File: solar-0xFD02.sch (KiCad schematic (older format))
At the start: 25 parts, among them J1 Solar, J2 BAT, J3 ESP32, Q1 MOSFET, U1 CN3801

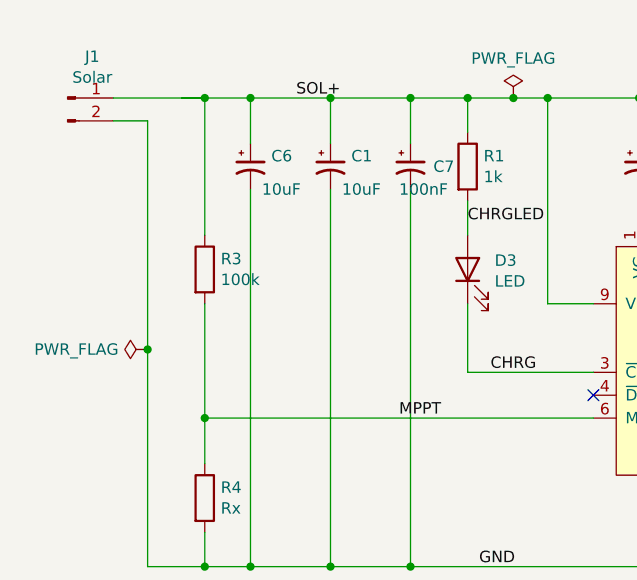
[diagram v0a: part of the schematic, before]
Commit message: Cleanup
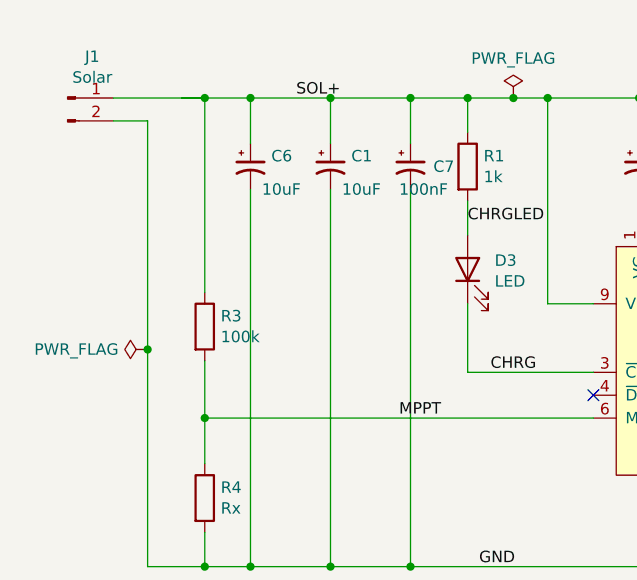
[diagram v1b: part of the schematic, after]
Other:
- moved on the sheet: R3
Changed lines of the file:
@@
 L Device:R R3
 U 1 1 600DC61D
-P 1900 2000
-F 0 "R3" H 1970 2046 50  0000 L CNN
-F 1 "100k" H 1970 1955 50  0000 L CNN
-F 2 "Resistor_SMD:R_1206_3216Metric_Pad1.30x1.75mm_HandSolder" V 1830 2000 50  0001 C CNN
-F 3 "~" H 1900 2000 50  0001 C CNN
-	1    1900 2000
+P 1900 2250
+F 0 "R3" H 1970 2296 50  0000 L CNN
+F 1 "100k" H 1970 2205 50  0000 L CNN
+F 2 "Resistor_SMD:R_1206_3216Metric_Pad1.30x1.75mm_HandSolder" V 1830 2250 50  0001 C CNN
+F 3 "~" H 1900 2250 50  0001 C CNN
+	1    1900 2250
 	1    0    0    -1
 $EndComp
@@
 	3400 1250 3250 1250
 Wire Wire Line
-	1900 1850 1900 1250
+	1900 2100 1900 1250
 Connection ~ 1900 1250
 Wire Wire Line
@@
 	3600 2650 1900 2650
 Wire Wire Line
-	1900 2650 1900 2150
+	1900 2650 1900 2400
 $Comp
 L Device:R R4
